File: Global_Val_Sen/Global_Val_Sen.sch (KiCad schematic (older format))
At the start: 63 parts, among them IC2 DW01A, Q1 FS8205A, Q2 IRF7303, U1 CPU1, U2 TP4056

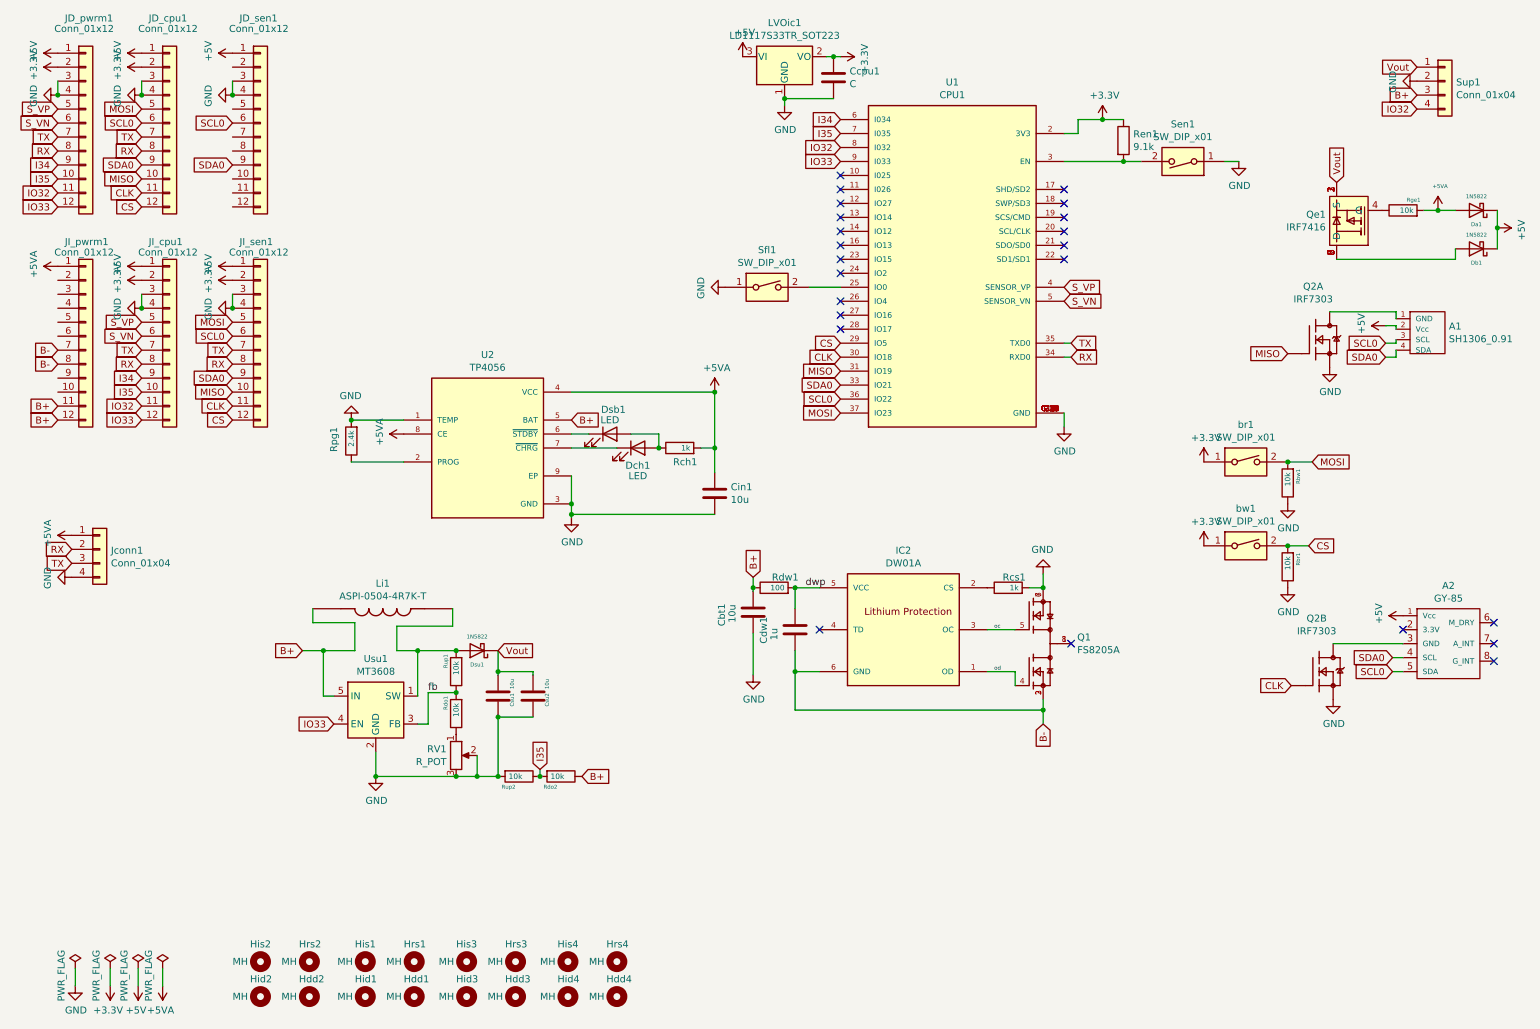
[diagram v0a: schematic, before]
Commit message: actualizacion sensor Cod &PCB
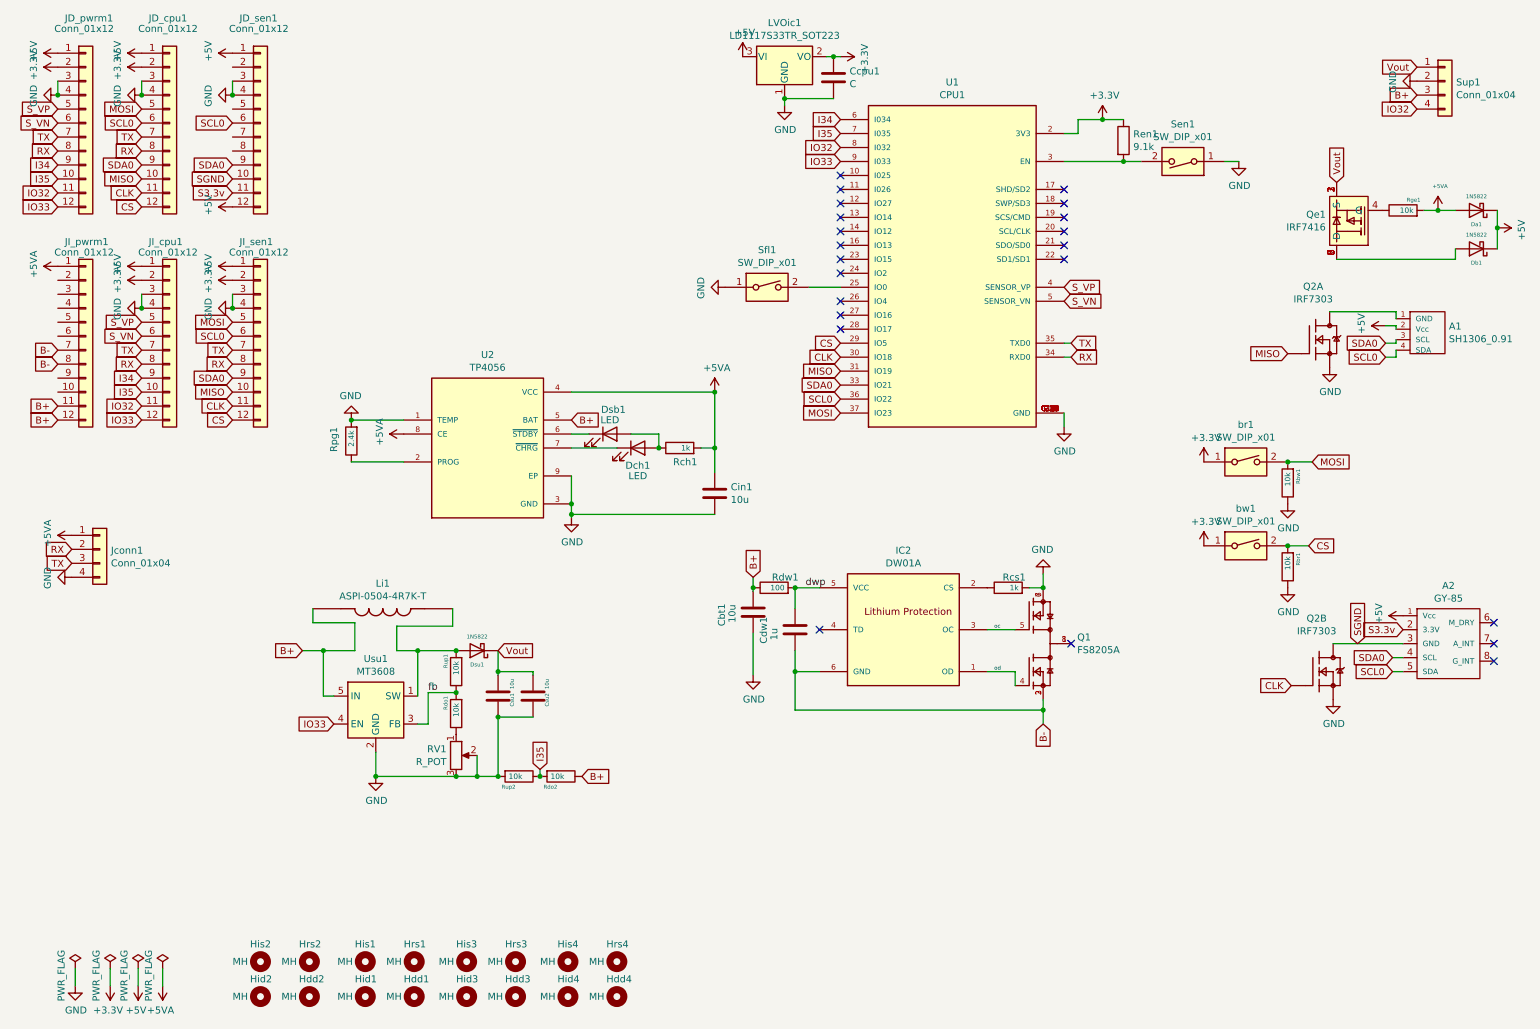
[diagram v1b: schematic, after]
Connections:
- net +5V: now also JD_sen1.12 (Pin_12)
- net SCL0: now also A1.4 (SDA); no longer A1.3 (SCL)
- net SDA0: now also A1.3 (SCL); no longer A1.4 (SDA)
- net SGND: now reaches JD_sen1.10 (Pin_10)
- net SGND: now also A2.3 (GND), Q2.5, Q2.6
- net S3.3v: now reaches JD_sen1.11 (Pin_11)
- net S3.3v: now also A2.2 (3.3V)
- no-connect marks 23 -> 22
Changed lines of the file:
@@
 	1    0    0    -1
 $EndComp
-Text GLabel 10100 2975 0    50   Input ~ 0
+Text GLabel 10100 2875 0    50   Input ~ 0
 SDA0
 Wire Wire Line
@@
 Wire Wire Line
 	10175 2775 10175 2750
-Text GLabel 10100 2875 0    50   Input ~ 0
+Text GLabel 10100 2975 0    50   Input ~ 0
 SCL0
 Wire Wire Line
@@
 Wire Wire Line
 	10175 2700 10175 2650
-Text GLabel 10150 5125 0    50   Input ~ 0
-SDA0
-Text GLabel 10150 5225 0    50   Input ~ 0
-SCL0
 Wire Wire Line
 	10225 5125 10150 5125
@@
 	0    -1   -1   0
 $EndComp
-NoConn ~ 10225 4925
 Wire Wire Line
 	10225 5025 9725 5025
@@
 NoConn ~ 10875 5025
 NoConn ~ 10875 4875
+Text GLabel 10150 5125 0    50   Input ~ 0
+SDA0
+Text GLabel 10150 5225 0    50   Input ~ 0
+SCL0
+$Comp
+L power:+5V #PWR0129
+U 1 1 6360CDDA
+P 1850 1900
+F 0 "#PWR0129" H 1850 1750 50  0001 C CNN
+F 1 "+5V" H 1865 2073 50  0000 C CNN
+F 2 "" H 1850 1900 50  0001 C CNN
+F 3 "" H 1850 1900 50  0001 C CNN
+	1    1850 1900
+	0    -1   -1   0
+$EndComp
+Text GLabel 9900 5025 1    50   Input ~ 0
+SGND
+Text GLabel 1850 1700 0    50   Input ~ 0
+SGND
+Text GLabel 10225 4925 0    50   Input ~ 0
+S3.3v
+Text GLabel 1850 1800 0    50   Input ~ 0
+S3.3v
 $EndSCHEMATC
